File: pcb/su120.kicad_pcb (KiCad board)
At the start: 2 copper layers, 99.2 x 99.2 mm, 324 parts, among them J1 MJ-4PP-9, J2 Conn_01x03, J3 Conn_01x08, J4 Conn_01x08, J5 Conn_01x03, J6 MJ-4PP-9, SW1 SW_Push, SW10 SW_Push, SW11 SW_Push, SW12 SW_Push, SW13 SW_Push, SW14 SW_Push, SW15 SW_Push, SW16 SW_Push, SW17 SW_Push, SW18 SW_Push, SW19 SW_Push, SW2 SW_Push, SW20 SW_Push, SW3 SW_Push, SW4 SW_Push, SW5 SW_Push, SW6 SW_Push, SW7 SW_Push, SW8 SW_Push, SW9 SW_Push, U1 ProMicro

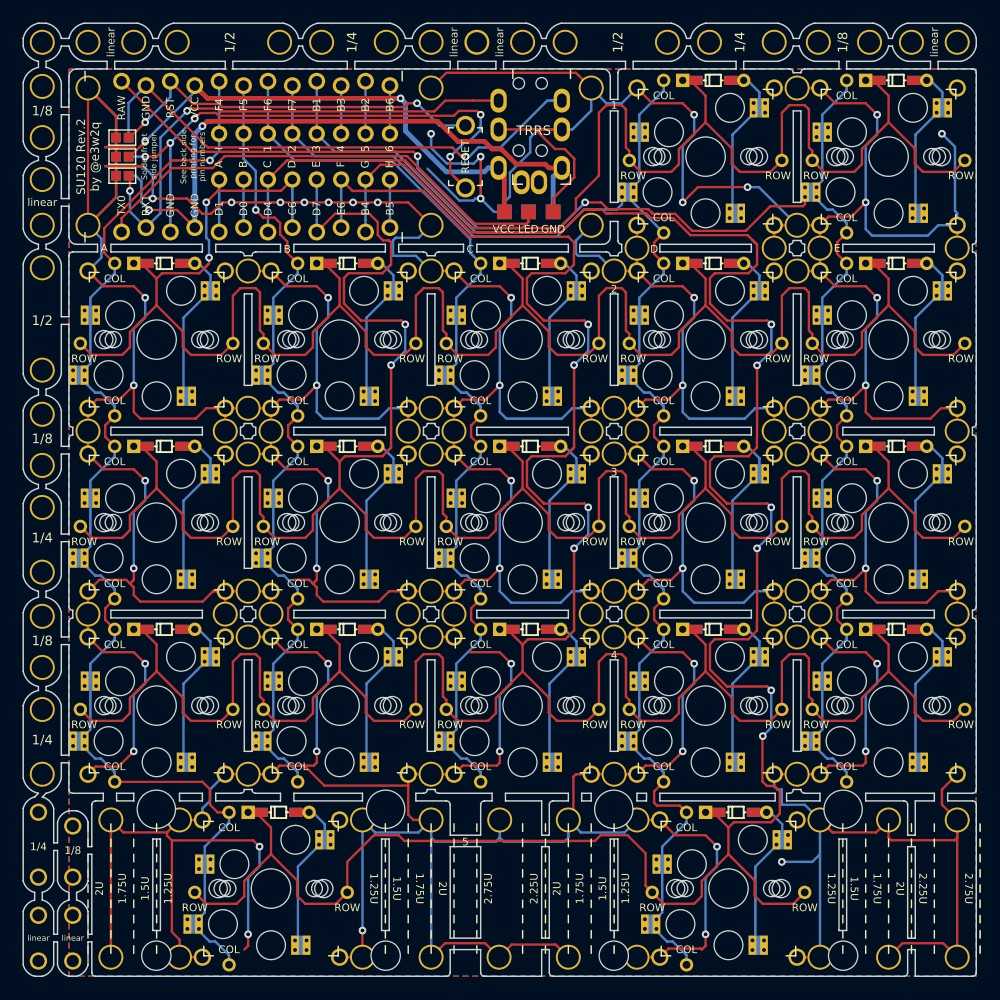
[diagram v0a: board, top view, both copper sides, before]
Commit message: Rev.3
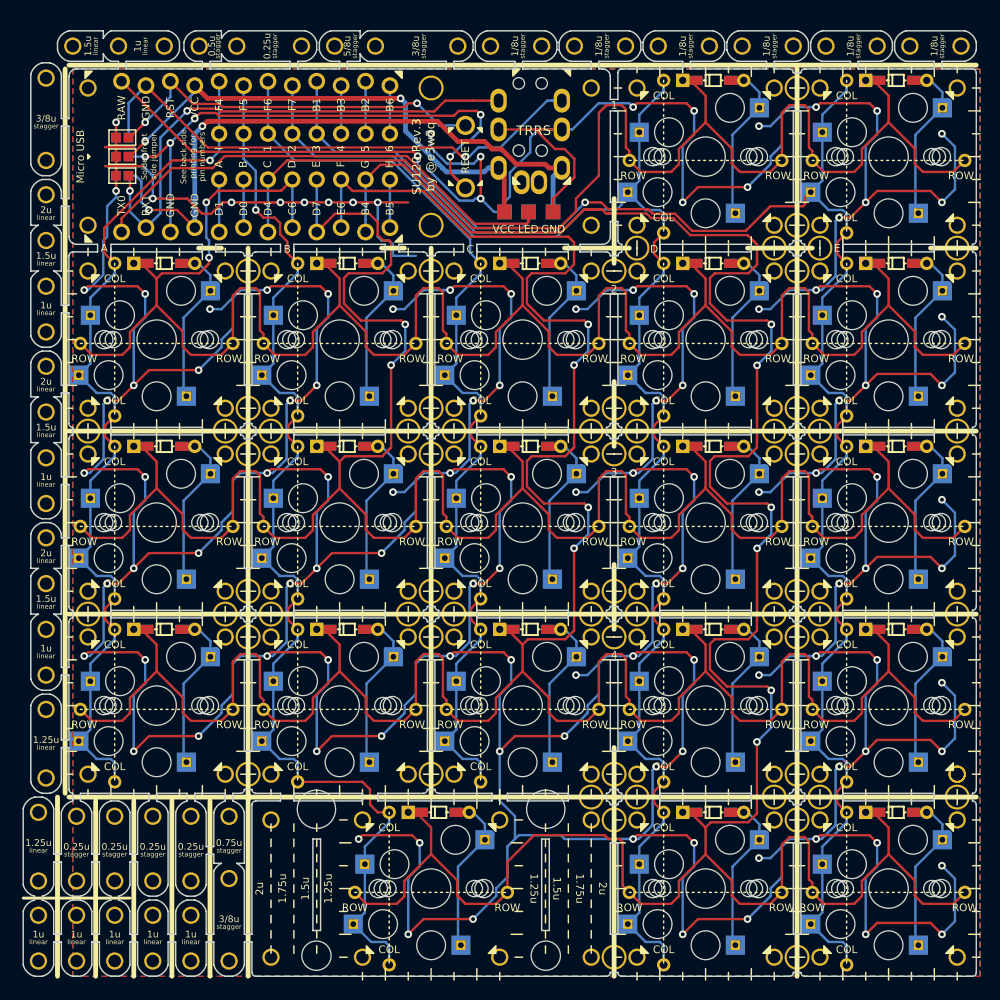
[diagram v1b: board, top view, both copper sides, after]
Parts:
- removed the ? at (39.7, 69.1)
- removed the ? at (39.7, 59.4)
- removed the ? at (39.7, 73.8)
- removed the ? at (39.7, 64.7)
- removed the ? at (39.7, 93.5)
- removed the ? at (39.7, 98.8)
- removed the ? at (39.7, 109.9)
- removed the ? at (39.7, 114.5)
- removed the ? at (39.7, 103.2)
- removed the ? at (39.7, 119.9)
- removed the ? at (39.3, 145.7)
- removed the ? at (134.9, 59.5)
- removed the ? at (115.9, 59.5)
- removed the ? at (58.7, 78.6)
- removed the ? at (77.8, 78.6)
- removed the ? at (96.8, 78.6)
- removed the ? at (115.9, 78.6)
- removed the ? at (134.9, 78.6)
- removed the ? at (134.9, 97.6)
- removed the ? at (115.9, 97.6)
- removed the ? at (96.8, 97.6)
- removed the ? at (39.3, 150.4)
- removed the ? at (77.8, 97.6)
- removed the ? at (58.7, 97.6)
- removed the ? at (58.7, 116.7)
- removed the ? at (77.8, 116.7)
- removed the ? at (96.8, 116.7)
- removed the ? at (115.9, 116.7)
- removed the ? at (134.9, 116.7)
- removed the ? at (118.3, 135.7)
- removed the ? at (70.6, 135.7)
- removed the ? at (39.3, 134.9)
- removed the ? at (80.2, 54.8)
- removed the ? at (84.9, 54.8)
- removed the ? at (89.7, 54.8)
- removed the ? at (49.2, 54.8)
- removed the ? at (44.5, 54.8)
- removed the ? at (75.5, 54.8)
- removed the ? at (68.8, 54.8)
- removed the ? at (53.7, 54.8)
- removed the ? at (64.4, 54.8)
- removed the ? at (39.3, 141.7)
- removed the ? at (94.1, 54.8)
- removed the ? at (104.8, 54.8)
- removed the ? at (115.9, 54.8)
- removed the ? at (125.8, 54.8)
- removed the ? at (120.5, 54.8)
- removed the ? at (130.2, 54.8)
- removed the ? at (134.9, 54.8)
- removed the ? at (109.2, 54.8)
- removed the ? at (39.7, 54.8)
- removed the ? at (39.7, 78.3)
- removed the ? at (42.9, 136.4)
- removed the ? at (39.7, 88.9)
- removed the ? at (39.7, 124.2)
- removed the ? at (39.7, 131.0)
- removed the ? at (42.9, 150.4)
- removed the ? at (42.9, 141.7)
- removed the ? at (42.9, 145.7)
- removed the ? at (111.1, 142.9)
- removed H100, H101, H102, H103, H104, H105, H106, H107, H108, H109, H110, H111, H112, H141, H142, H143, H144, H145, H146, H147, H148, H149, H150, H151, H152, H49, H50, H51, H52, H53, H54, H55, H56, H57, H58, H59, H60, H61, H62, H63, H64, H65, H66, H67, H68, H69, H70, H71, H72, H73, H74, H75, H76, H77, H78, H79, H80, H81, H82, H83, H84, H85, H86, H87, H88, H89, H90, H91, H92, H93, H94, H95, H96, H97, H98, H99: MountingHole_Pad, #footprint:M2_Pad
- removed H153, H154, H155, H156, H158, H159, H160, H161, H162, H163, H164, H165, H166, H167, H168, H169, H170, H171, H172, H173, H174, H175, H176, H177, H178, H179, H180, H181, H182, H183, H184, H185, H186, H187, H188, H189, H190, H191, H192, H193, H194, H195, H196, H197, H198, H199, H200, H201, H202, H203, H204, H205, H206, H207, H208, H209: MountingHole_Pad, #footprint:M1.4_tapping_Pad
- added ?: , #footprint:M2, F.Cu at (99.2, 78.6)
- added ?: , #footprint:M1.4_tapping_Pad, F.Cu at (39.3, 142.1)
- added ?: , #footprint:M1.4_tapping_Pad, F.Cu at (39.3, 134.9)
- added ?: , #footprint:M1.4_tapping_Pad, F.Cu at (70.1, 55.2)
- added ?: , #footprint:M1.4_tapping_Pad, F.Cu at (82.9, 55.2)
- added ?: , #footprint:M1.4_tapping_Pad, F.Cu at (74.4, 55.2)
- added ?: , #footprint:M1.4_tapping_Pad, F.Cu at (40.1, 58.5)
- added ?: , #footprint:M1.4_tapping_Pad, F.Cu at (40.1, 67.1)
- added ?: , #footprint:M1.4_tapping_Pad, F.Cu at (44.5, 59.5)
- added ?: , #footprint:M1.4_tapping_Pad, F.Cu at (96.8, 59.5)
- added ?: , #footprint:M1.4_tapping_Pad, F.Cu at (101.6, 59.5)
- added ?: , #footprint:M2, F.Cu at (118.3, 73.8)
- added ?: , #footprint:M1.4_tapping_Pad, F.Cu at (115.9, 59.5)
- added ?: , #footprint:M1.4_tapping_Pad, F.Cu at (120.7, 59.5)
- added ?: , #footprint:M1.4_tapping_Pad, F.Cu at (134.9, 59.5)
- added ?: , #footprint:M1.4_tapping_Pad, F.Cu at (134.9, 73.8)
- added ?: , #footprint:M1.4_tapping_Pad, F.Cu at (120.7, 73.8)
- added ?: , #footprint:M1.4_tapping_Pad, F.Cu at (115.9, 73.8)
- added ?: , #footprint:M1.4_tapping_Pad, F.Cu at (101.6, 73.8)
- added ?: , #footprint:M1.4_tapping_Pad, F.Cu at (96.8, 73.8)
- added ?: , #footprint:M1.4_tapping_Pad, F.Cu at (44.5, 73.8)
- added ?: , #footprint:M1.4_tapping_Pad, F.Cu at (44.5, 78.6)
- added ?: , #footprint:M2, F.Cu at (115.9, 76.2)
- added ?: , #footprint:M1.4_tapping_Pad, F.Cu at (58.7, 78.6)
- added ?: , #footprint:M1.4_tapping_Pad, F.Cu at (63.5, 78.6)
- added ?: , #footprint:M1.4_tapping_Pad, F.Cu at (77.8, 78.6)
- added ?: , #footprint:M1.4_tapping_Pad, F.Cu at (82.5, 78.6)
- added ?: , #footprint:M1.4_tapping_Pad, F.Cu at (96.8, 78.6)
- added ?: , #footprint:M1.4_tapping_Pad, F.Cu at (101.6, 78.6)
- added ?: , #footprint:M1.4_tapping_Pad, F.Cu at (115.9, 78.6)
- added ?: , #footprint:M1.4_tapping_Pad, F.Cu at (120.7, 78.6)
- added ?: , #footprint:M1.4_tapping_Pad, F.Cu at (134.9, 78.6)
- added ?: , #footprint:M1.4_tapping_Pad, F.Cu at (134.9, 92.9)
- added ?: , #footprint:M2, F.Cu at (118.3, 78.6)
- added ?: , #footprint:M1.4_tapping_Pad, F.Cu at (120.7, 92.9)
- added ?: , #footprint:M1.4_tapping_Pad, F.Cu at (115.9, 92.9)
- added ?: , #footprint:M1.4_tapping_Pad, F.Cu at (101.6, 92.9)
- added ?: , #footprint:M1.4_tapping_Pad, F.Cu at (96.8, 92.9)
- added ?: , #footprint:M1.4_tapping_Pad, F.Cu at (82.5, 92.9)
- added ?: , #footprint:M1.4_tapping_Pad, F.Cu at (77.8, 92.9)
- added ?: , #footprint:M1.4_tapping_Pad, F.Cu at (63.5, 92.9)
- added ?: , #footprint:M1.4_tapping_Pad, F.Cu at (58.7, 92.9)
- added ?: , #footprint:M1.4_tapping_Pad, F.Cu at (44.5, 92.9)
- added ?: , #footprint:M1.4_tapping_Pad, F.Cu at (44.5, 97.6)
- added ?: , #footprint:M2, F.Cu at (120.7, 76.2)
- added ?: , #footprint:M1.4_tapping_Pad, F.Cu at (58.7, 97.6)
- added ?: , #footprint:M1.4_tapping_Pad, F.Cu at (63.5, 97.6)
- added ?: , #footprint:M1.4_tapping_Pad, F.Cu at (77.8, 97.6)
- added ?: , #footprint:M1.4_tapping_Pad, F.Cu at (82.5, 97.6)
- added ?: , #footprint:M1.4_tapping_Pad, F.Cu at (96.8, 97.6)
- added ?: , #footprint:M1.4_tapping_Pad, F.Cu at (101.6, 97.6)
- added ?: , #footprint:M1.4_tapping_Pad, F.Cu at (115.9, 97.6)
- added ?: , #footprint:M1.4_tapping_Pad, F.Cu at (120.7, 97.6)
- added ?: , #footprint:M1.4_tapping_Pad, F.Cu at (134.9, 97.6)
- added ?: , #footprint:M1.4_tapping_Pad, F.Cu at (134.9, 111.9)
- added ?: , #footprint:M2, F.Cu at (134.9, 76.2)
- added ?: , #footprint:M1.4_tapping_Pad, F.Cu at (120.7, 111.9)
- added ?: , #footprint:M1.4_tapping_Pad, F.Cu at (115.9, 111.9)
- added ?: , #footprint:M1.4_tapping_Pad, F.Cu at (101.6, 111.9)
- added ?: , #footprint:M1.4_tapping_Pad, F.Cu at (96.8, 111.9)
- added ?: , #footprint:M1.4_tapping_Pad, F.Cu at (82.5, 111.9)
- added ?: , #footprint:M1.4_tapping_Pad, F.Cu at (77.8, 111.9)
- added ?: , #footprint:M1.4_tapping_Pad, F.Cu at (63.5, 111.9)
- added ?: , #footprint:M1.4_tapping_Pad, F.Cu at (58.7, 111.9)
- added ?: , #footprint:M1.4_tapping_Pad, F.Cu at (44.5, 111.9)
- added ?: , #footprint:M1.4_tapping_Pad, F.Cu at (44.5, 116.7)
- added ?: , #footprint:M2, F.Cu at (134.9, 95.2)
- added ?: , #footprint:M1.4_tapping_Pad, F.Cu at (58.7, 116.7)
- added ?: , #footprint:M1.4_tapping_Pad, F.Cu at (63.5, 116.7)
- added ?: , #footprint:M1.4_tapping_Pad, F.Cu at (77.8, 116.7)
- added ?: , #footprint:M1.4_tapping_Pad, F.Cu at (82.5, 116.7)
- added ?: , #footprint:M1.4_tapping_Pad, F.Cu at (96.8, 116.7)
- added ?: , #footprint:M1.4_tapping_Pad, F.Cu at (101.6, 116.7)
- added ?: , #footprint:M1.4_tapping_Pad, F.Cu at (115.9, 116.7)
- added ?: , #footprint:M1.4_tapping_Pad, F.Cu at (120.7, 116.7)
- added ?: , #footprint:M1.4_tapping_Pad, F.Cu at (134.9, 116.7)
- added ?: , #footprint:M1.4_tapping_Pad, F.Cu at (134.9, 131.0)
- added ?: , #footprint:M2, F.Cu at (118.3, 92.9)
- added ?: , #footprint:M1.4_tapping_Pad, F.Cu at (120.7, 131.0)
- added ?: , #footprint:M1.4_tapping_Pad, F.Cu at (115.9, 131.0)
- added ?: , #footprint:M1.4_tapping_Pad, F.Cu at (101.6, 131.0)
- added ?: , #footprint:M1.4_tapping_Pad, F.Cu at (96.8, 131.0)
- added ?: , #footprint:M1.4_tapping_Pad, F.Cu at (82.5, 131.0)
- added ?: , #footprint:M1.4_tapping_Pad, F.Cu at (77.8, 131.0)
- added ?: , #footprint:M1.4_tapping_Pad, F.Cu at (63.5, 131.0)
- added ?: , #footprint:M1.4_tapping_Pad, F.Cu at (58.7, 131.0)
- added ?: , #footprint:M1.4_tapping_Pad, F.Cu at (44.5, 131.0)
- added ?: , #footprint:M1.4_tapping_Pad, F.Cu at (63.5, 135.7)
- added ?: , #footprint:M2, F.Cu at (120.7, 95.2)
- added ?: , #footprint:M1.4_tapping_Pad, F.Cu at (73.0, 135.7)
- added ?: , #footprint:M1.4_tapping_Pad, F.Cu at (87.3, 135.7)
- added ?: , #footprint:M1.4_tapping_Pad, F.Cu at (96.8, 135.7)
- added ?: , #footprint:M1.4_tapping_Pad, F.Cu at (101.6, 135.7)
- added ?: , #footprint:M1.4_tapping_Pad, F.Cu at (115.9, 135.7)
- added ?: , #footprint:M1.4_tapping_Pad, F.Cu at (120.7, 135.7)
- added ?: , #footprint:M1.4_tapping_Pad, F.Cu at (134.9, 135.7)
- added ?: , #footprint:M1.4_tapping_Pad, F.Cu at (134.9, 150.0)
- added ?: , #footprint:M1.4_tapping_Pad, F.Cu at (120.7, 150.0)
- added ?: , #footprint:M1.4_tapping_Pad, F.Cu at (115.9, 150.0)
- added ?: , #footprint:M2, F.Cu at (118.3, 97.6)
- added ?: , #footprint:M1.4_tapping_Pad, F.Cu at (101.6, 150.0)
- added ?: , #footprint:M1.4_tapping_Pad, F.Cu at (96.8, 150.0)
- added ?: , #footprint:M1.4_tapping_Pad, F.Cu at (87.3, 150.0)
- added ?: , #footprint:M1.4_tapping_Pad, F.Cu at (73.0, 150.0)
- added ?: , #footprint:M1.4_tapping_Pad, F.Cu at (63.5, 150.0)
- added ?: , #footprint:M1.4_tapping_Pad, F.Cu at (43.3, 142.1)
- added ?: , #footprint:M1.4_tapping_Pad, F.Cu at (43.3, 135.3)
- added ?: , #footprint:M1.4_tapping_Pad, F.Cu at (130.0, 55.2)
- added ?: , #footprint:M1.4_tapping_Pad, F.Cu at (135.3, 55.2)
- added ?: , #footprint:M1.4_tapping_Pad, F.Cu at (91.7, 55.2)
- added ?: , #footprint:M2, F.Cu at (134.9, 133.3)
- added ?: , #footprint:M2, F.Cu at (115.9, 95.2)
- added ?: , #footprint:M1.4_tapping_Pad, F.Cu at (86.4, 55.2)
- added ?: , #footprint:M1.4_tapping_Pad, F.Cu at (121.3, 55.2)
- added ?: , #footprint:M1.4_tapping_Pad, F.Cu at (112.5, 55.2)
- added ?: , #footprint:M1.4_tapping_Pad, F.Cu at (117.9, 55.2)
- added ?: , #footprint:M1.4_tapping_Pad, F.Cu at (126.6, 55.2)
- added ?: , #footprint:M1.4_tapping_Pad, F.Cu at (95.1, 55.2)
- added ?: , #footprint:M1.4_tapping_Pad, F.Cu at (100.4, 55.2)
- added ?: , #footprint:M1.4_tapping_Pad, F.Cu at (109.1, 55.2)
- added ?: , #footprint:M1.4_tapping_Pad, F.Cu at (103.8, 55.2)
- added ?: , #footprint:M1.4_tapping_Pad, F.Cu at (43.3, 150.4)
- added ?: , #footprint:M2, F.Cu at (99.2, 92.9)
- added ?: , #footprint:M1.4_tapping_Pad, F.Cu at (43.3, 145.7)
- added ?: , #footprint:M2, F.Cu at (101.6, 95.2)
- added ?: , #footprint:M2, F.Cu at (99.2, 97.6)
- added ?: , #footprint:M2, F.Cu at (96.8, 95.2)
- added ?: , #footprint:M2, F.Cu at (80.2, 92.9)
- added ?: , #footprint:M2, F.Cu at (82.5, 95.2)
- added ?: , #footprint:M2, F.Cu at (80.2, 97.6)
- added ?: , #footprint:M2, F.Cu at (77.8, 95.2)
- added ?: , #footprint:M2, F.Cu at (61.1, 92.9)
- added ?: , #footprint:M2, F.Cu at (80.2, 59.5)
- added ?: , #footprint:M2, F.Cu at (63.5, 95.2)
- added ?: , #footprint:M2, F.Cu at (61.1, 97.6)
- added ?: , #footprint:M2, F.Cu at (58.7, 95.2)
- added ?: , #footprint:M2, F.Cu at (44.5, 95.2)
- added ?: , #footprint:M2, F.Cu at (44.5, 114.3)
- added ?: , #footprint:M2, F.Cu at (58.7, 114.3)
- added ?: , #footprint:M2, F.Cu at (61.1, 111.9)
- added ?: , #footprint:M2, F.Cu at (63.5, 114.3)
- added ?: , #footprint:M2, F.Cu at (61.1, 116.7)
- added ?: , #footprint:M2, F.Cu at (77.8, 114.3)
- added ?: , #footprint:M2, F.Cu at (80.2, 73.8)
- added ?: , #footprint:M2, F.Cu at (80.2, 111.9)
- added ?: , #footprint:M2, F.Cu at (82.5, 114.3)
- added ?: , #footprint:M2, F.Cu at (80.2, 116.7)
- added ?: , #footprint:M2, F.Cu at (96.8, 114.3)
- added ?: , #footprint:M2, F.Cu at (99.2, 111.9)
- added ?: , #footprint:M2, F.Cu at (101.6, 114.3)
- added ?: , #footprint:M2, F.Cu at (99.2, 116.7)
- added ?: , #footprint:M2, F.Cu at (115.9, 114.3)
- added ?: , #footprint:M2, F.Cu at (118.3, 111.9)
- added ?: , #footprint:M2, F.Cu at (120.7, 114.3)
- added ?: , #footprint:M2, F.Cu at (115.9, 133.3)
- added ?: , #footprint:M2, F.Cu at (118.3, 116.7)
- added ?: , #footprint:M2, F.Cu at (134.9, 114.3)
- added ?: , #footprint:M2, F.Cu at (118.3, 150.0)
- added ?: , #footprint:M2, F.Cu at (120.7, 133.3)
- added ?: , #footprint:M2, F.Cu at (118.3, 135.7)
- added ?: , #footprint:M2, F.Cu at (118.3, 131.0)
- added ?: , #footprint:M2, F.Cu at (101.6, 133.3)
- added ?: , #footprint:M2, F.Cu at (96.8, 133.3)
- added ?: , #footprint:M2, F.Cu at (99.2, 150.0)
- added ?: , #footprint:M2, F.Cu at (99.2, 135.7)
- added ?: , #footprint:M2, F.Cu at (118.3, 59.5)
- added ?: , #footprint:M2, F.Cu at (99.2, 131.0)
- added ?: , #footprint:M2, F.Cu at (80.2, 131.0)
- added ?: , #footprint:M2, F.Cu at (61.1, 131.0)
- added ?: , #footprint:M1.4_tapping_Pad, F.Cu at (42.9, 55.2)
- added ?: , #footprint:M1.4_tapping_Pad, F.Cu at (52.4, 55.2)
- added ?: , #footprint:M1.4_tapping_Pad, F.Cu at (47.6, 55.2)
- added ?: , #footprint:M1.4_tapping_Pad, F.Cu at (59.1, 141.8)
- added ?: , #footprint:M1.4_tapping_Pad, F.Cu at (39.3, 145.7)
- added ?: , #footprint:M1.4_tapping_Pad, F.Cu at (39.3, 150.4)
- added ?: , #footprint:M1.4_tapping_Pad, F.Cu at (47.2, 150.4)
- added ?: , #footprint:M2, F.Cu at (61.1, 78.6)
- added ?: , #footprint:M1.4_tapping_Pad, F.Cu at (47.2, 142.1)
- added ?: , #footprint:M1.4_tapping_Pad, F.Cu at (47.2, 145.7)
- added ?: , #footprint:M1.4_tapping_Pad, F.Cu at (47.2, 135.3)
- added ?: , #footprint:M1.4_tapping_Pad, F.Cu at (51.2, 142.1)
- added ?: , #footprint:M1.4_tapping_Pad, F.Cu at (51.2, 145.7)
- added ?: , #footprint:M1.4_tapping_Pad, F.Cu at (51.2, 135.3)
- added ?: , #footprint:M1.4_tapping_Pad, F.Cu at (51.2, 150.4)
- added ?: , #footprint:M1.4_tapping_Pad, F.Cu at (55.2, 142.1)
- added ?: , #footprint:M1.4_tapping_Pad, F.Cu at (55.2, 145.7)
- added ?: , #footprint:M1.4_tapping_Pad, F.Cu at (55.2, 135.3)
- added ?: , #footprint:M2, F.Cu at (80.2, 78.6)
- added ?: , #footprint:M1.4_tapping_Pad, F.Cu at (55.2, 150.4)
- added ?: , #footprint:M1.4_tapping_Pad, F.Cu at (59.1, 135.4)
- added ?: , #footprint:M1.4_tapping_Pad, F.Cu at (59.1, 150.4)
- added ?: , #footprint:M1.4_tapping_Pad, F.Cu at (40.1, 80.2)
- added ?: , #footprint:M1.4_tapping_Pad, F.Cu at (40.1, 75.4)
- added ?: , #footprint:M1.4_tapping_Pad, F.Cu at (40.1, 84.9)
- added ?: , #footprint:M1.4_tapping_Pad, F.Cu at (40.1, 70.6)
- added ?: , #footprint:M1.4_tapping_Pad, F.Cu at (40.1, 88.5)
- added ?: , #footprint:M1.4_tapping_Pad, F.Cu at (40.1, 98.0)
- added ?: , #footprint:M1.4_tapping_Pad, F.Cu at (40.1, 102.8)
- added ?: , #footprint:M2, F.Cu at (101.6, 76.2)
- added ?: , #footprint:M1.4_tapping_Pad, F.Cu at (40.1, 93.3)
- added ?: , #footprint:M1.4_tapping_Pad, F.Cu at (56.0, 55.2)
- added ?: , #footprint:M1.4_tapping_Pad, F.Cu at (59.9, 55.2)
- added ?: , #footprint:M1.4_tapping_Pad, F.Cu at (66.7, 55.2)
- added ?: , #footprint:M1.4_tapping_Pad, F.Cu at (40.1, 106.4)
- added ?: , #footprint:M1.4_tapping_Pad, F.Cu at (40.1, 111.1)
- added ?: , #footprint:M1.4_tapping_Pad, F.Cu at (40.1, 120.7)
- added ?: , #footprint:M1.4_tapping_Pad, F.Cu at (40.1, 115.9)
- added ?: , #footprint:M1.4_tapping_Pad, F.Cu at (40.1, 131.4)
- added ?: , #footprint:M1.4_tapping_Pad, F.Cu at (40.1, 124.2)
- added D20: D, #footprint:diode_TH_SMD, F.Cu at (125.8, 134.9)
- added H210: MountingHole_Pad, #footprint:1pin_conn, F.Cu at (123.4, 134.9)
- added H211: MountingHole_Pad, #footprint:1pin_conn, F.Cu at (123.4, 150.8)
- added H212: MountingHole_Pad, #footprint:1pin_conn, F.Cu at (119.9, 143.3)
- added H213: MountingHole_Pad, #footprint:1pin_conn, F.Cu at (135.7, 143.3)
- added SW21: SW_Push, #footprint:CherryMX_MidHeight_Choc_Hotswap_rev4, F.Cu at (127.8, 142.9)
- SW1, SW10, SW11, SW12, SW13, SW14, SW15, SW16, SW17, SW19, SW2, SW20, SW3, SW4, SW5, SW6, SW7, SW8, SW9: footprint #footprint:CherryMX_MidHeight_Choc_Hotswap_rev2 -> #footprint:CherryMX_MidHeight_Choc_Hotswap_rev4
- moved ? 16.7 mm to (80.2, 142.9)
- moved D16 16.7 mm to (78.2, 134.9)
- moved H45 16.7 mm to (72.2, 143.3)
- moved H46 16.7 mm to (88.1, 143.3)
- moved SW16 16.7 mm to (80.2, 142.9)
- moved H41 16.7 mm to (75.8, 134.9)
- moved H43 16.7 mm to (75.8, 150.8)
- moved H42 2.38 mm to (104.4, 134.9)
- moved H44 2.38 mm to (104.4, 150.8)
- moved D17 2.38 mm to (106.8, 134.9)
- moved H47 2.38 mm to (100.8, 143.3)
- moved H48 2.38 mm to (116.7, 143.3)
- moved SW17 2.38 mm to (108.7, 142.9)
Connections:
- H41 pad 1: X1 -> X2
- H43 pad 1: X1 -> X2
- J1 pad A: Net-(J1-PadA) -> (no net)
- J6 pad A: Net-(J6-PadA) -> (no net)
- SW16 pad 1: X1 -> X2
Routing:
- net GND: track 1208.9 -> 978.4 mm, vias 52 -> 115
- net X2: track 87.2 -> 120.6 mm
- net X1: track 127.4 -> 95.9 mm
- net X5: track 153.9 -> 180.2 mm
- net Y5: track 252.8 -> 277.5 mm
- net Net-(D20-Pad2): track 0.00 -> 18.2 mm
- net X3: track 99.7 -> 101.5 mm
- net (no net): track 0.00 -> 1.68 mm
- net X4: track 160.0 -> 161.5 mm
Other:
- board size 99.2 x 99.2 mm -> 99.2 x 98.4 mm
- board text added: "0.25u"
- board text added: "0.5u"
- board text added: "0.75u"
- board text added: "1.25u"
- board text added: "1.5u"
- board text added: "1/8u"
- board text added: "1u"
- board text added: "2u"
- board text added: "3/8u"
- board text added: "5/8u"
- board text added: "SU120 Rev.3 by @e3w2q"
- board text added: "stagger"
- board text removed: "1/2"
- board text removed: "1/4"
- board text removed: "1/8"
- board text removed: "SU120 Rev.2 by @e3w2q"
